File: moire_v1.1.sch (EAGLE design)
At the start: 137 parts, among them IC1 TLC59281DBQ, IC11 LM4040B25, IC2 ROF-78E3.3-0.5SMD, IC3 4051PW, IC4 LM324PW, IC7 LD2981ABU33, IC9 LM324PW, J1 PJ301_THONKICONN6, J10 PJ301_THONKICONN6, J11 PJ301_THONKICONN6, J12 PJ301_THONKICONN6, J2 PJ301_THONKICONN6, J3 PJ301_THONKICONN6, J4 PJ301_THONKICONN6, J5 PJ301_THONKICONN6, J6 PJ301_THONKICONN6, J7 PJ301_THONKICONN6, J8 PJ301_THONKICONN6, J9 PJ301_THONKICONN6, Q2 8MHz, Q5 MMBT3904, Q6 MMBT3904, Q7 MMBT3904, U1 STM32F303K8T6, U2 MCP6004_SMD, U4 TL074_SMD

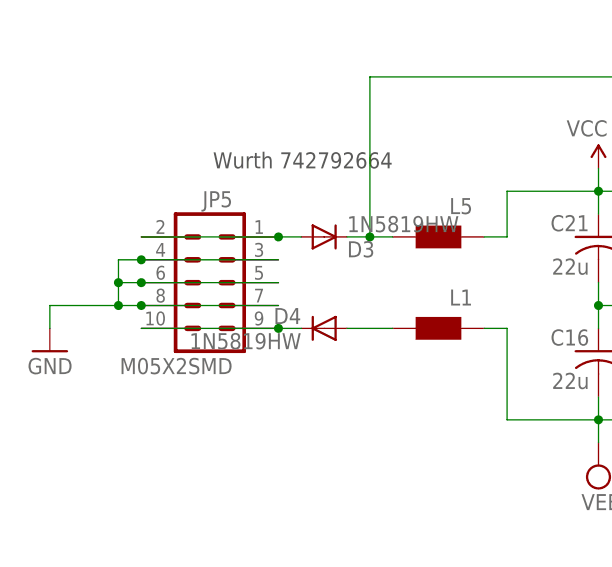
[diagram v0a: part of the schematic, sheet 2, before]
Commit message: update brd
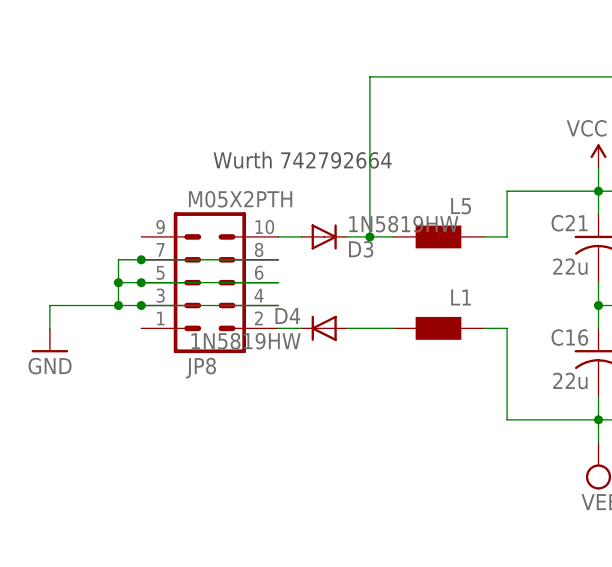
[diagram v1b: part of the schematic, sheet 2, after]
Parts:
- removed JP5: M05X2SMD, og-header:M05X2SMD
- added JP8: M05X2PTH, og-header:M05X2PTH
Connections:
- new net N$15: JP8.9
- new net N$17: JP8.1
- net GND: now also JP8.3, JP8.4, JP8.5, JP8.6, JP8.7, JP8.8; no longer JP5.3, JP5.4, JP5.5, JP5.6, JP5.7, JP5.8
- net N$18: now also JP8.10; no longer JP5.1, JP5.2
- net N$96: now also JP8.2; no longer JP5.10, JP5.9
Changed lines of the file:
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@@
 <part name="D3" library="diode" deviceset="DIODE-" device="SOD123" value="1N5819HW"/>
 <part name="D4" library="diode" deviceset="DIODE-" device="SOD123" value="1N5819HW"/>
-<part name="JP5" library="og-header" deviceset="M05X2" device="SMD"/>
 <part name="L5" library="wuerth-elektronik" deviceset="WE-CBF" device="_0603"/>
 <part name="L1" library="wuerth-elektronik" deviceset="WE-CBF" device="_0603"/>
@@
 <part name="P+2" library="SparkFun" deviceset="VCC" device=""/>
 <part name="IC4" library="og-linear" deviceset="TL074" device="PW" value="LM324PW"/>
+<part name="JP8" library="og-header" deviceset="M05X2" device="PTH" value="M05X2PTH"/>
 </parts>
 <sheets>
@@
 <attribute name="VALUE" x="-73.66" y="-15.0114" size="1.778" layer="96" rot="MR0"/>
 </instance>
-<instance part="JP5" gate="G$1" x="-83.82" y="-7.62" rot="MR0">
-<attribute name="VALUE" x="-81.28" y="-17.78" size="1.778" layer="96" rot="MR0"/>
-<attribute name="NAME" x="-81.28" y="0.762" size="1.778" layer="95" rot="MR0"/>
-</instance>
 <instance part="L5" gate="G$1" x="-58.42" y="-5.08" rot="MR0">
 <attribute name="VALUE" x="-54.61" y="-6.35" size="1.778" layer="96" rot="MR0"/>
@@
 <attribute name="NAME" x="74.676" y="-22.225" size="1.778" layer="95"/>
 <attribute name="VALUE" x="74.676" y="-27.051" size="1.778" layer="96"/>
+</instance>
+<instance part="JP8" gate="G$1" x="-83.82" y="-7.62" rot="MR180">
+<attribute name="VALUE" x="-86.36" y="2.54" size="1.778" layer="96" rot="MR180"/>
+<attribute name="NAME" x="-86.36" y="-16.002" size="1.778" layer="95" rot="MR180"/>
 </instance>
 </instances>
@@
 <junction x="-93.98" y="-7.62"/>
 <junction x="-93.98" y="-10.16"/>
+<pinref part="GND73" gate="1" pin="GND"/>
+<pinref part="JP8" gate="G$1" pin="8"/>
+<pinref part="JP8" gate="G$1" pin="6"/>
+<pinref part="JP8" gate="G$1" pin="4"/>
+<pinref part="JP8" gate="G$1" pin="7"/>
+<junction x="-91.44" y="-5.08"/>
+<pinref part="JP8" gate="G$1" pin="5"/>
+<junction x="-91.44" y="-7.62"/>
+<pinref part="JP8" gate="G$1" pin="3"/>
 <junction x="-91.44" y="-10.16"/>
-<junction x="-91.44" y="-7.62"/>
-<junction x="-91.44" y="-5.08"/>
-<pinref part="GND73" gate="1" pin="GND"/>
-<pinref part="JP5" gate="G$1" pin="8"/>
-<pinref part="JP5" gate="G$1" pin="6"/>
-<pinref part="JP5" gate="G$1" pin="4"/>
-<pinref part="JP5" gate="G$1" pin="7"/>
-<pinref part="JP5" gate="G$1" pin="5"/>
-<pinref part="JP5" gate="G$1" pin="3"/>
 </segment>
 <segment>
@@
 <net name="N$18" class="0">
 <segment>
-<wire x1="-76.2" y1="-2.54" x2="-91.44" y2="-2.54" width="0.1524" layer="91"/>
-<wire x1="-76.2" y1="-2.54" x2="-73.66" y2="-2.54" width="0.1524" layer="91"/>
-<junction x="-76.2" y="-2.54"/>
-<pinref part="JP5" gate="G$1" pin="2"/>
-<pinref part="JP5" gate="G$1" pin="1"/>
 <pinref part="D3" gate="G$1" pin="A"/>
+<wire x1="-73.66" y1="-2.54" x2="-76.2" y2="-2.54" width="0.1524" layer="91"/>
+<pinref part="JP8" gate="G$1" pin="10"/>
 </segment>
 </net>
 <net name="N$96" class="0">
 <segment>
-<wire x1="-76.2" y1="-12.7" x2="-91.44" y2="-12.7" width="0.1524" layer="91"/>
-<wire x1="-76.2" y1="-12.7" x2="-73.66" y2="-12.7" width="0.1524" layer="91"/>
-<junction x="-76.2" y="-12.7"/>
-<pinref part="JP5" gate="G$1" pin="10"/>
-<pinref part="JP5" gate="G$1" pin="9"/>
 <pinref part="D4" gate="G$1" pin="C"/>
+<wire x1="-73.66" y1="-12.7" x2="-76.2" y2="-12.7" width="0.1524" layer="91"/>
+<pinref part="JP8" gate="G$1" pin="2"/>
 </segment>
 </net>
@@
 </segment>
 </net>
+<net name="N$15" class="0">
+<segment>
+<wire x1="-91.44" y1="-2.54" x2="-91.44" y2="-2.54" width="0.1524" layer="91"/>
+<pinref part="JP8" gate="G$1" pin="9"/>
+</segment>
+</net>
+<net name="N$17" class="0">
+<segment>
+<wire x1="-91.44" y1="-12.7" x2="-91.44" y2="-12.7" width="0.1524" layer="91"/>
+<pinref part="JP8" gate="G$1" pin="1"/>
+</segment>
+</net>
